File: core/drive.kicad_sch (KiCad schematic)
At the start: 31 parts, among them Q3 BSS84, Q4 MMBT3904, Q5 MMBT3904, Q6 MMBT3906, Q7 MMBT3906, Q8 MMBT3904, U3 TL072, U4 TL072

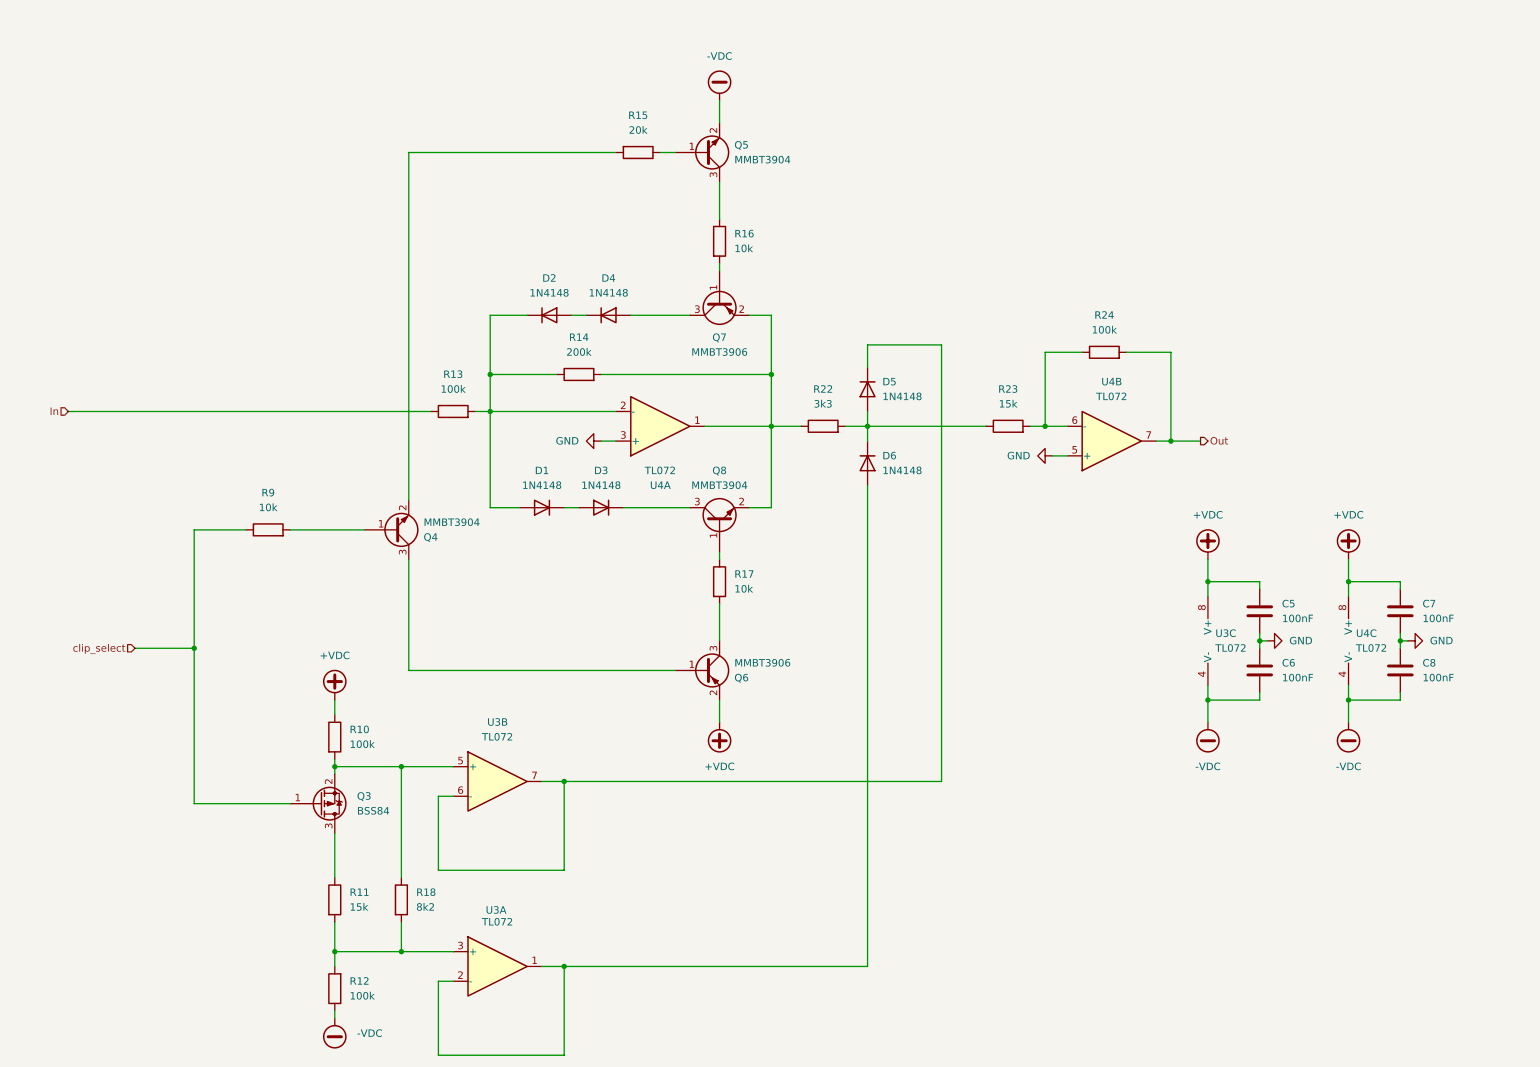
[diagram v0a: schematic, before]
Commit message: Fixes for v1.1
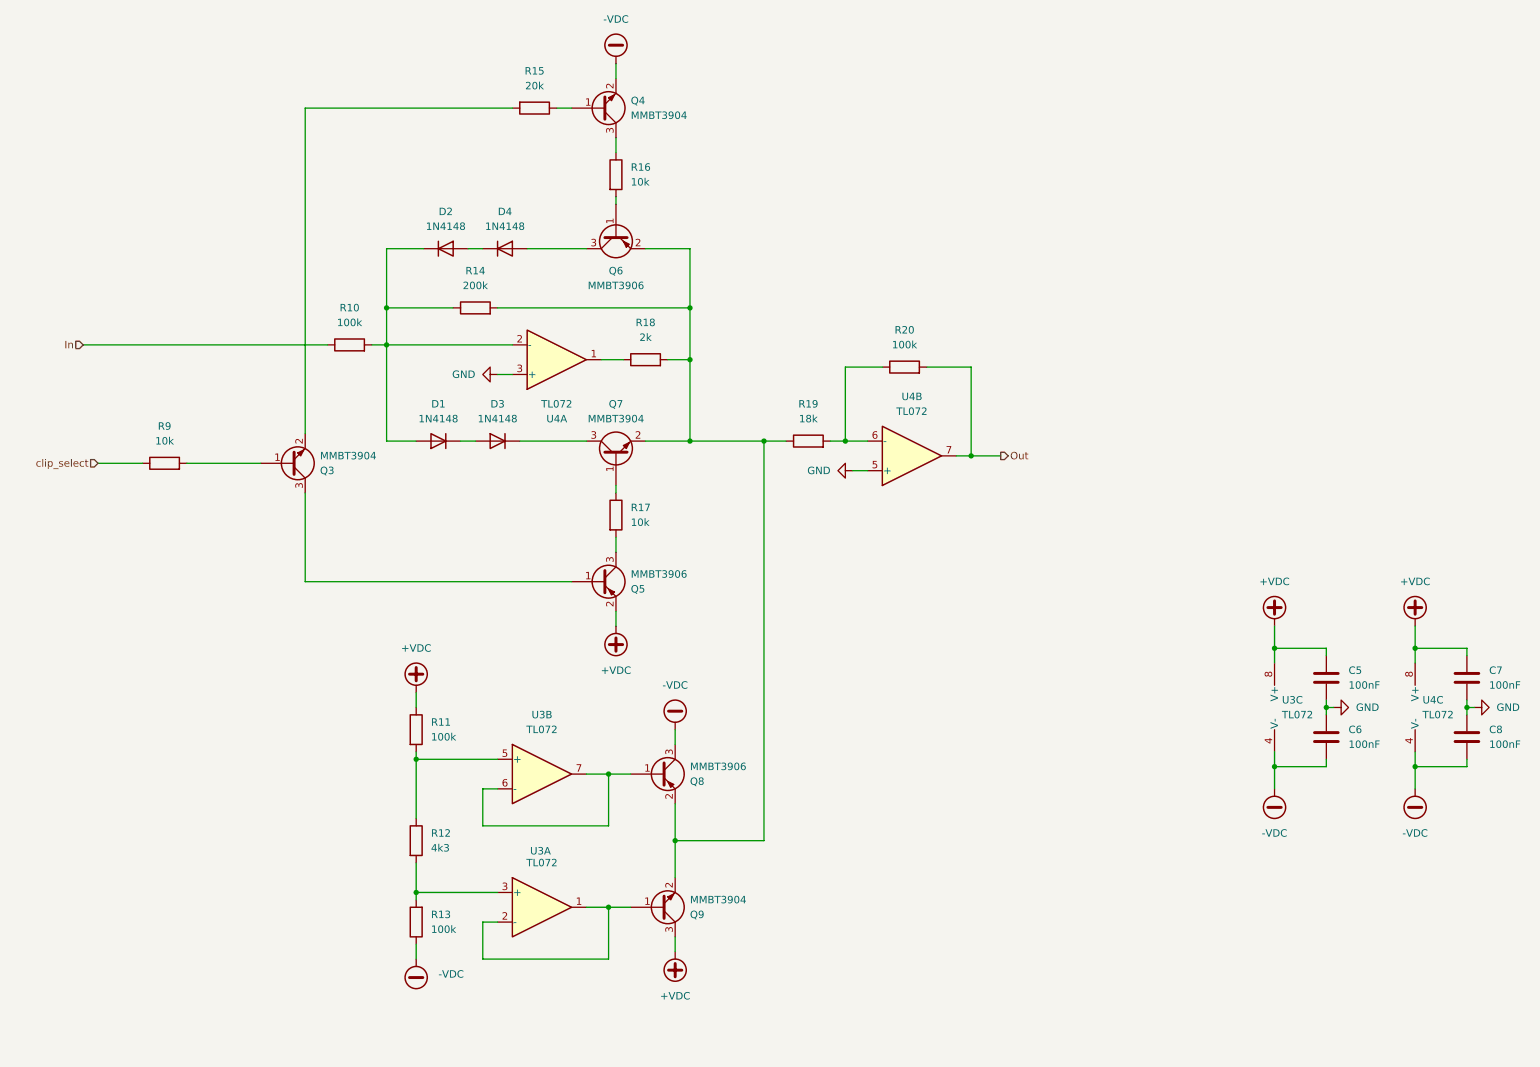
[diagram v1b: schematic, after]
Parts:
- removed D5, D6: 1N4148, Diode_SMD:D_SOD-323_HandSoldering, symbol Device:D
- removed Q3: BSS84, Package_TO_SOT_SMD:SOT-23, symbol Transistor_FET:BSS84
- removed R11: 15k, Resistor_SMD:R_0603_1608Metric, symbol Device:R
- added Q8: MMBT3906, Package_TO_SOT_SMD:SOT-23, symbol Transistor_BJT:MMBT3906
- added Q9: MMBT3904, Package_TO_SOT_SMD:SOT-23, symbol Transistor_BJT:MMBT3904
- R12: renamed from R18; value 8k2 -> 4k3
- R18: renamed from R22; value 3k3 -> 2k
- R19: renamed from R23; value 15k -> 18k
- renumbered Q4 to Q3, Q5 to Q4, Q6 to Q5, Q7 to Q6, Q8 to Q7, R13 to R10, R10 to R11, R12 to R13, R24 to R20
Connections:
- net +VDC: now also Q9.3 (C)
- net -VDC: now also Q8.3 (C)
- net at R18.2, R19.1: now also Q6.2 (E), Q7.2 (E), R14.2, Q8.2 (E), Q9.2 (E)
- net at U3.6 (-), U3.7: now also Q8.1 (B)
- net at U3.1, U3.2 (-): now also Q9.1 (B)
- new net: R18.1, U4.1
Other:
- moved on the sheet: C5, C6, C7, C8, D1, D2, D3, D4, Q3, Q4, Q5, Q6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
